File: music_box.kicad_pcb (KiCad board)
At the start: 2 copper layers, 34 x 36 mm, 39 parts, among them J1 USB_C_Receptacle, J2 UART, P1 ICSPforPICKit, Q1 IRLML6402, Q2 IRLML6402, SW1 SW_Push, U1 CH340E, U2 PIC16(L)F18324, U3 24FC256, U4 TC118SS, U5 TLV61225

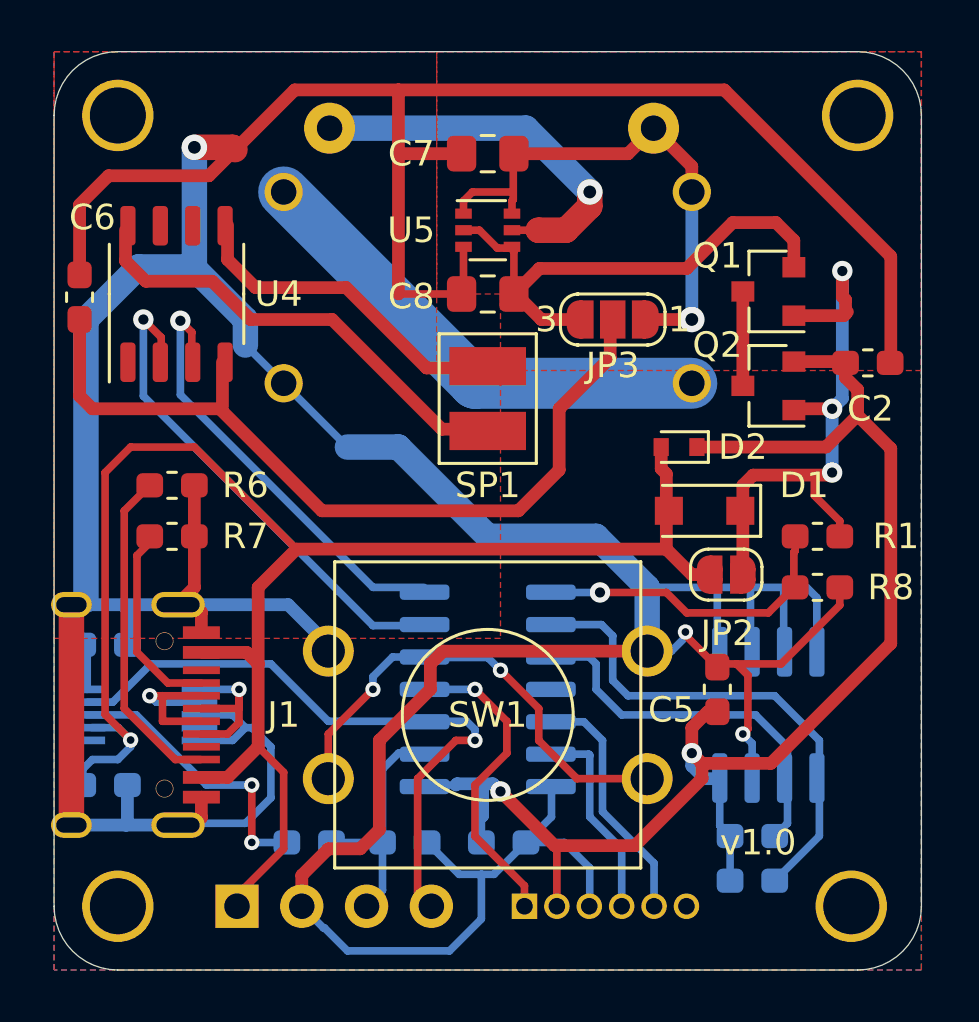
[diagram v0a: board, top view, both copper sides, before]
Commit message: ver2
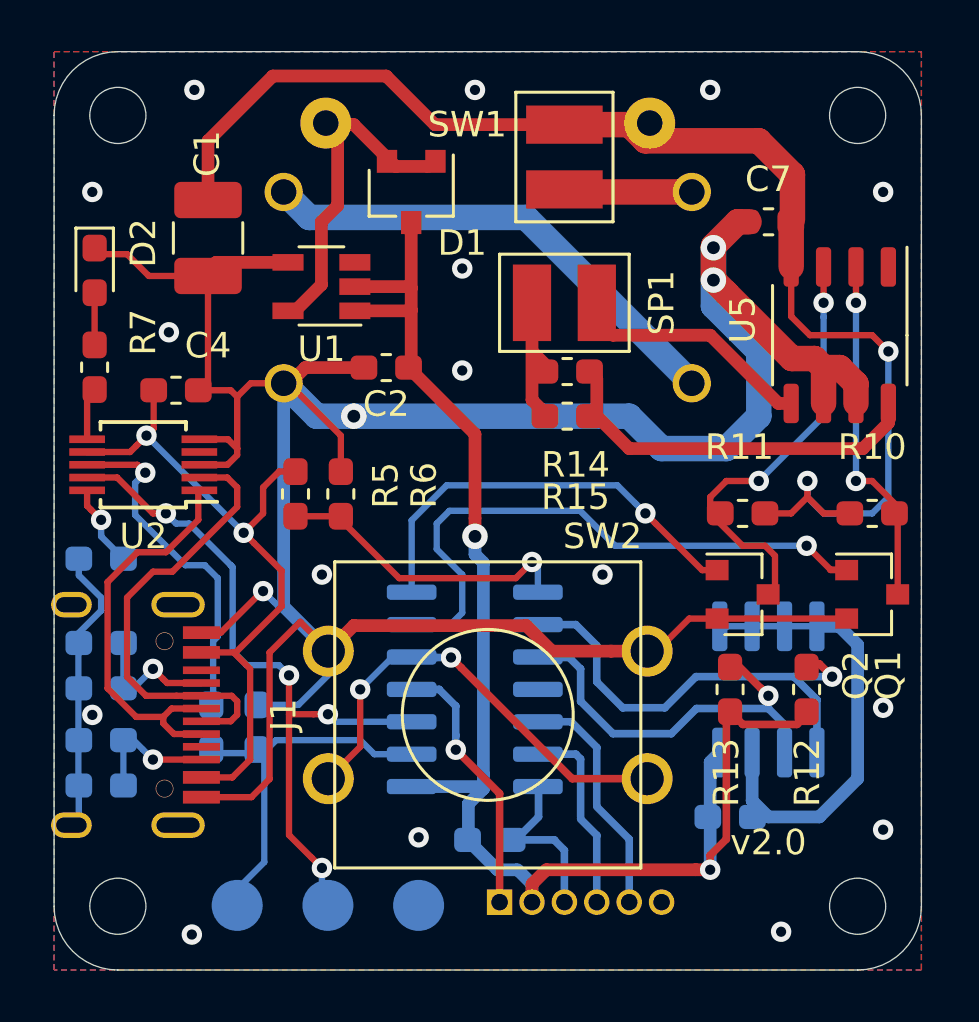
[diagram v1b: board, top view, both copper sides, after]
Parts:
- removed the C2 at (51.9, 32.2)
- removed J2: UART, Connector_PinHeader_2.54mm:PinHeader_1x04_P2.54mm_Vertical
- removed JP2: D1_Bridge, Jumper:SolderJumper-2_P1.3mm_Open_RoundedPad1.0x1.5mm
- removed JP3: SP_SORCE, Jumper:SolderJumper-3_P1.3mm_Open_RoundedPad1.0x1.5mm_NumberLabels
- removed the R6 at (24.6, 37.0)
- removed the U5 at (37.0, 27.0)
- added R1: 10k, Resistor_SMD:R_0603_1608Metric_Pad1.05x0.95mm_HandSolder, B.Cu at (21.8, 48.8)
- added R10: 10k, Resistor_SMD:R_0603_1608Metric_Pad1.05x0.95mm_HandSolder, F.Cu at (52.1, 38.1)
- added R11: 10k, Resistor_SMD:R_0603_1608Metric_Pad1.05x0.95mm_HandSolder, F.Cu at (47.0, 38.1)
- added R14: 47, Resistor_SMD:R_0603_1608Metric_Pad1.05x0.95mm_HandSolder, F.Cu at (40.1, 32.5)
- added R15: 47, Resistor_SMD:R_0603_1608Metric_Pad1.05x0.95mm_HandSolder, F.Cu at (40.1, 34.3)
- added R2: 10k, Resistor_SMD:R_0603_1608Metric_Pad1.05x0.95mm_HandSolder, B.Cu at (21.8, 47.0)
- added R3: 10k, Resistor_SMD:R_0603_1608Metric_Pad1.05x0.95mm_HandSolder, B.Cu at (21.8, 45.0)
- added R4: 10k, Resistor_SMD:R_0603_1608Metric_Pad1.05x0.95mm_HandSolder, B.Cu at (21.8, 43.2)
- added SW1: POWER, fues-connect:2.54-2pin-lay, F.Cu at (40.0, 24.1)
- added TP1: tp_PC2MC, TestPoint:TestPoint_Pad_D2.0mm, B.Cu at (27.2, 53.5)
- added TP2: tp_MC2PC, TestPoint:TestPoint_Pad_D2.0mm, B.Cu at (30.7, 53.5)
- added TP3: tp_GND, TestPoint:TestPoint_Pad_D2.0mm, B.Cu at (34.3, 53.5)
- added U1: HT77XXA_SOT-25, Package_TO_SOT_SMD:TSOT-23-5, F.Cu at (30.5, 29.2)
- C1: renamed from C7; value C -> 47u; footprint Capacitor_SMD:C_0805_2012Metric_Pad1.15x1.40mm_HandSolder -> Capacitor_SMD:C_1210_3225Metric_Pad1.42x2.65mm_HandSolder
- C2: renamed from C8; value C -> 22u; footprint Capacitor_SMD:C_0805_2012Metric_Pad1.15x1.40mm_HandSolder -> Capacitor_SMD:C_0603_1608Metric_Pad1.05x0.95mm_HandSolder
- C3: renamed from C1; value 0.1u -> 0.1u 1608
- C4: renamed from C3; value 0.1u -> 0.1u 1608; moved to F.Cu
- C5: value 0.1u -> 0.1u 1608; moved to B.Cu
- C6: renamed from C4; value 0.1u -> 0.1u 1608
- C7: renamed from C6; value 0.1u -> 0.1u 1608
- D1: value GS1010FL -> RB411D; footprint Diode_SMD:D_SOD-123F -> Package_TO_SOT_SMD:SC-59
- D2: value RB751S-40 -> LED NC; footprint Diode_SMD:D_SOD-523 -> Diode_SMD:D_0603_1608Metric_Pad1.05x0.95mm_HandSolder
- H1, H2, H3, H4: footprint fues-mounting_hole:M2-drillHole -> fues-mounting_hole:M2-drillHole_nosilk_nopad
- L1: value L -> 100uH
- Q1, Q2: value IRLML6402 -> 2n7002
- R12: renamed from R2; moved to F.Cu
- R13: renamed from R3; moved to F.Cu
- R7: value 5.1k -> 470 NC
- SP1: value buzzer -> sp
- U2: renamed from U1; moved to F.Cu
- moved C7 27.2 mm to (48.0, 26.7), turned to 180 degrees
- moved U5 26.1 mm to (50.8, 31.1), turned to 270 degrees
- moved D2 23.9 mm to (21.6, 28.6), turned to 270 degrees
- moved R5 20.5 mm to (29.5, 37.3), turned to 270 degrees
- moved R6 19.0 mm to (31.2, 37.3), turned to 90 degrees
- moved D1 17.0 mm to (34.0, 25.5), turned to 270 degrees
- moved C4 15.7 mm to (24.8, 33.3)
- moved Q1 12.6 mm to (52.1, 41.3), turned to 0 degrees
- moved C1 11.5 mm to (26.0, 27.3), turned to 270 degrees
- moved U2 9.81 mm to (23.5, 36.2)
- moved Q2 8.24 mm to (47.0, 41.3), turned to 0 degrees
- moved R12 7.80 mm to (49.5, 45.0), turned to 90 degrees
- moved R9 7.36 mm to (27.9, 46.5), turned to 90 degrees
- moved R7 7.29 mm to (21.6, 32.4), turned to 90 degrees
- moved R8 5.93 mm to (26.2, 46.5), turned to 270 degrees
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- renumbered BT2 to BT1, BT1 to BT2, R1 to R5, R8 to R6, R4 to R8, R5 to R9, SW1 to SW2, U2 to U3, U3 to U4, U4 to U5
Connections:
- net Net-(U2-Pad11) renamed /FLOATING
- BT1 pad 1: +BATT -> Net-(BT1-Pad1)
- C5 pad 1: VDD -> +3V3
- C6 pad 1: VDD -> +3V3
- C7 pad 1: Net-(C6-Pad1) -> +BATT
- D1 pad 2: +5V -> Net-(D1-Pad1)
- D2 pad 1: VDD -> GND
- D2 pad 2: +5V -> Net-(D2-Pad2)
- L1 pad 2: Net-(L1-Pad2) -> Net-(D1-Pad1)
- P1 pad 2: VDD -> +3V3
- Q1 pad 1: Net-(D1-Pad1) -> /SPD1
- Q1 pad 2: +3V3 -> GND
- Q1 pad 3: Net-(Q1-Pad3) -> /SPD1_1
- Q2 pad 1: Net-(D1-Pad1) -> /SPD2
- Q2 pad 2: VDD -> GND
- Q2 pad 3: Net-(Q1-Pad3) -> /SPD2_1
- R12 pad 1: VDD -> +3V3
- R13 pad 1: VDD -> +3V3
- R5 pad 1: Net-(D1-Pad1) -> +5V
- R7 pad 1: Net-(J1-PadA5) -> Net-(R7-Pad1)
- R7 pad 2: GND -> Net-(D2-Pad2)
- SP1 pad 1: Net-(SP1-Pad1) -> Net-(R14-Pad2)
- U2 pad 6: Net-(U1-Pad6) -> Net-(R7-Pad1)
- U3 pad 1: VDD -> +3V3
- U4 pad 8: VDD -> +3V3
- U5 pad 2: /SPD1 -> /SPD1_1
- U5 pad 3: /SPD2 -> /SPD2_1
- U5 pad 4: Net-(C6-Pad1) -> +BATT
- U5 pad 8: Net-(SP1-Pad1) -> Net-(R14-Pad1)
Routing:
- net GND: track 227.7 -> 156.6 mm, vias 3 -> 20
- net VDD: track 60.9 -> 0.00 mm, vias 2 -> 0
- net +5V: track 66.9 -> 27.6 mm, vias 1 -> 2
- net +3V3: track 20.3 -> 59.3 mm, vias 0 -> 2
- net Net-(C6-Pad1): track 32.9 -> 0.00 mm
- net +BATT: track 20.8 -> 52.5 mm, vias 1 -> 2
- net Net-(SP1-Pad1): track 18.3 -> 0.00 mm
- net /SPD2_1: track 0.00 -> 17.0 mm, vias 0 -> 2
- net Net-(L1-Pad2): track 15.3 -> 0.00 mm, vias 1 -> 0
- net Net-(R14-Pad1): track 0.00 -> 15.0 mm
- net /SPD1_1: track 0.00 -> 13.9 mm, vias 0 -> 2
- net /D-: track 6.60 -> 18.1 mm, vias 1 -> 0
- net Net-(D1-Pad1): track 23.3 -> 12.5 mm, vias 3 -> 0
- net /D+: track 6.56 -> 16.1 mm, vias 1 -> 0
- net Net-(J1-PadB5): track 13.0 -> 4.61 mm, vias 0 -> 1
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- removed copper zone on F.Cu, net +BATT
- removed copper zone on F.Cu, net VDD
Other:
- board text added: "kamibushiele.net"
- board text added: "v2.0"
- board text removed: "v1.0"
